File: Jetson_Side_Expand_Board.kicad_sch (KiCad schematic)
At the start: 13 parts, among them J1 Conn_01x12_Socket, J2 Conn_01x04_Socket, J3 Conn_01x04, J4 Conn_01x02_Pin, J5 Conn_01x02, J6 Conn_01x02_Pin, J7 Conn_01x02, J8 Conn_01x03_Pin, U1 TCAN332G

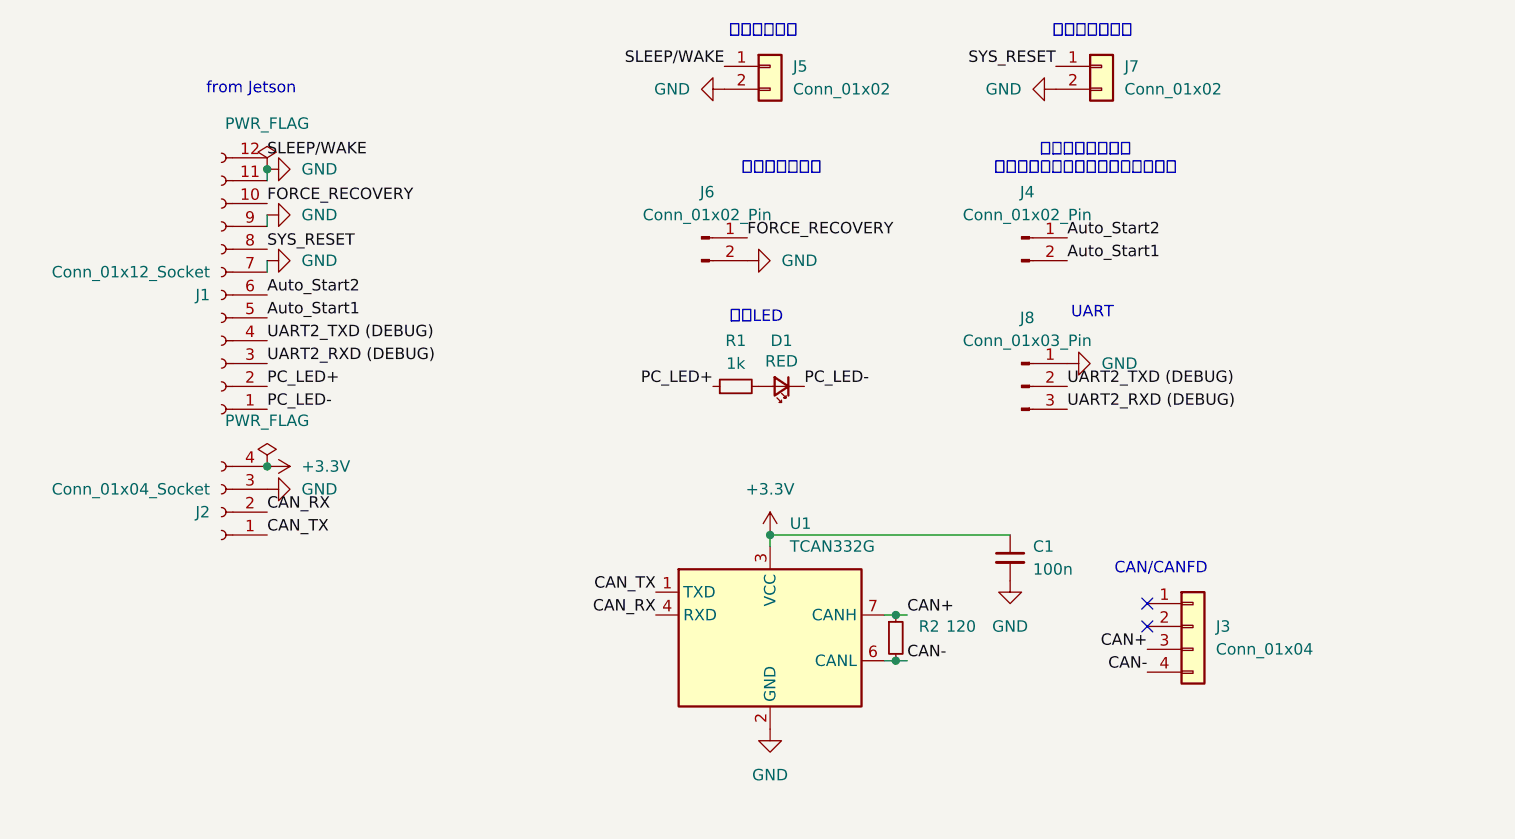
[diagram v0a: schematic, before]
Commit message: セラコンのGND
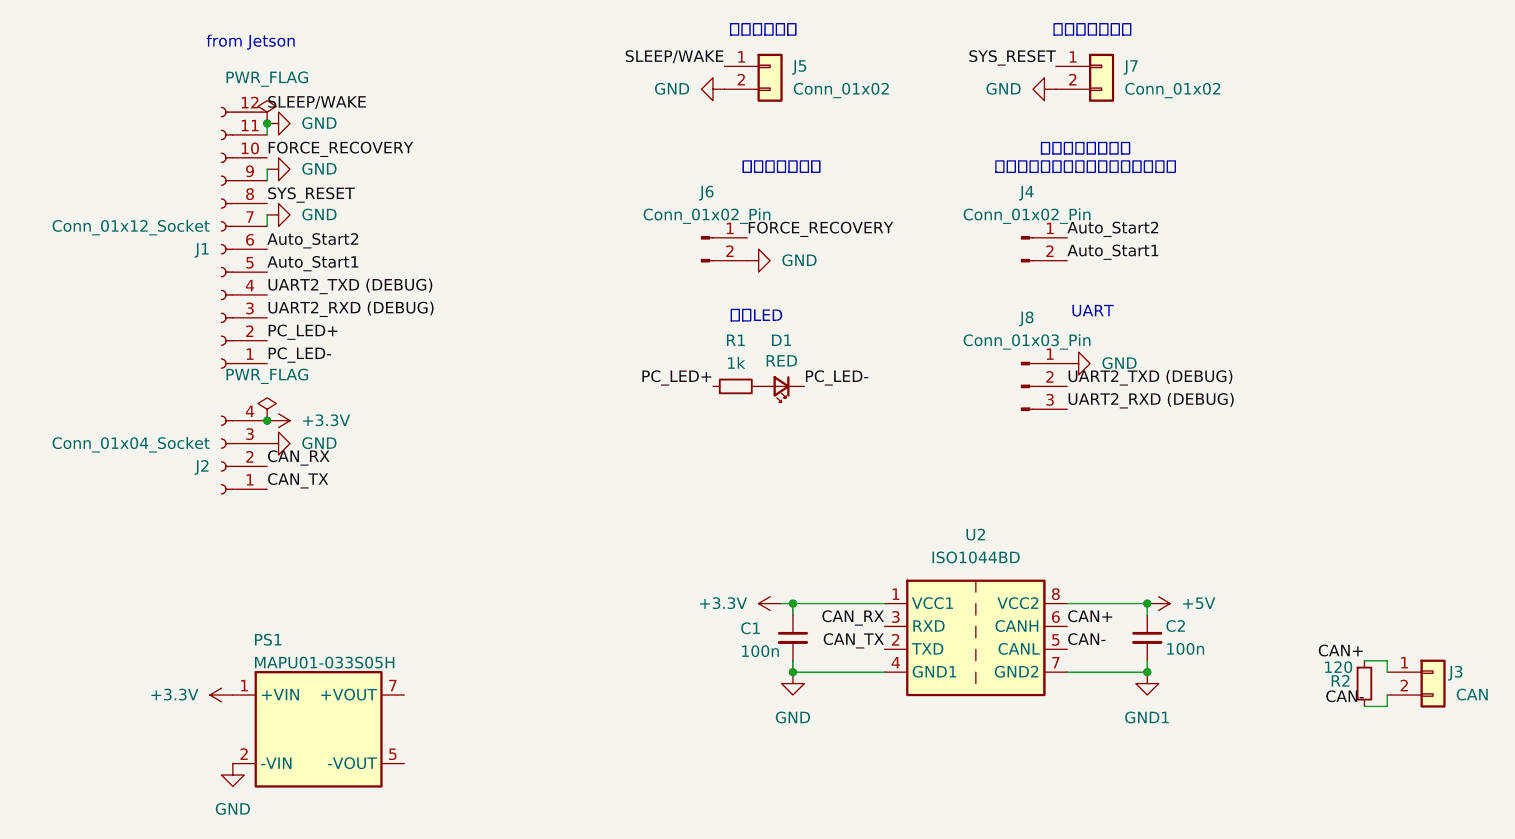
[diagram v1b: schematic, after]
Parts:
- removed J3: Conn_01x04, e-CON:e-CON_1×04, symbol Connector_Generic:Conn_01x04
- removed U1: TCAN332G, Package_SO:SOIC-8_3.9x4.9mm_P1.27mm, symbol Interface_CAN_LIN:TCAN332G
- added C2: 100n, symbol Device:C_Small
- added J3: CAN, symbol Connector_Generic:Conn_01x02
- added PS1: MAPU01-033S05H, MAPU01-033S05H:MAPU01033S033H, symbol MAPU01-033S05H:MAPU01-033S05H
- added U2: ISO1044BD, Package_SO:SOIC-8_3.9x4.9mm_P1.27mm, symbol Interface_CAN_LIN:ISO1044BD
- C1: footprint Capacitor_SMD:C_0603_1608Metric_Pad1.08x0.95mm_HandSolder -> (none)
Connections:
- net +3.3V: now also PS1.1 (+VIN), U2.1 (VCC1)
- net CAN+: now also J3.1 (Pin_1), U2.6 (CANH)
- net CAN-: now also J3.2 (Pin_2), U2.5 (CANL)
- net CAN_RX: now also U2.3 (RXD)
- net CAN_TX: now also U2.2 (TXD)
- net GND: now also PS1.2 (-VIN), U2.4 (GND1)
- new net +5V: C2.1, U2.8 (VCC2)
- new net GND1: C2.2, U2.7 (GND2)
- no-connect marks 2 -> 0
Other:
- note removed: "CAN/CANFD"
- moved on the sheet: J1, J2
